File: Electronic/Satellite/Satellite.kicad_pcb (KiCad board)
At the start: 4 copper layers, 40 x 40 mm, 119 parts, among them J3 Conn_01x10, J4 Conn_01x10, J5 Conn_01x10, SW1 TS-1088-AR02016, SW2 TS-1088-AR02016, U1 LAN8651B1-E/LMX, U2 AVRH10C221KT1R5YA8, U3 AVRH10C221KT1R5YA8, U4 SY8513FCC, U5 ABM8-272-T3_C20625731, U6 NCP1117ST33T3G, U7 RP2354A, U8 WS2812C-2020-V6, X1 ABM10-25.000MHZ-D30-T3

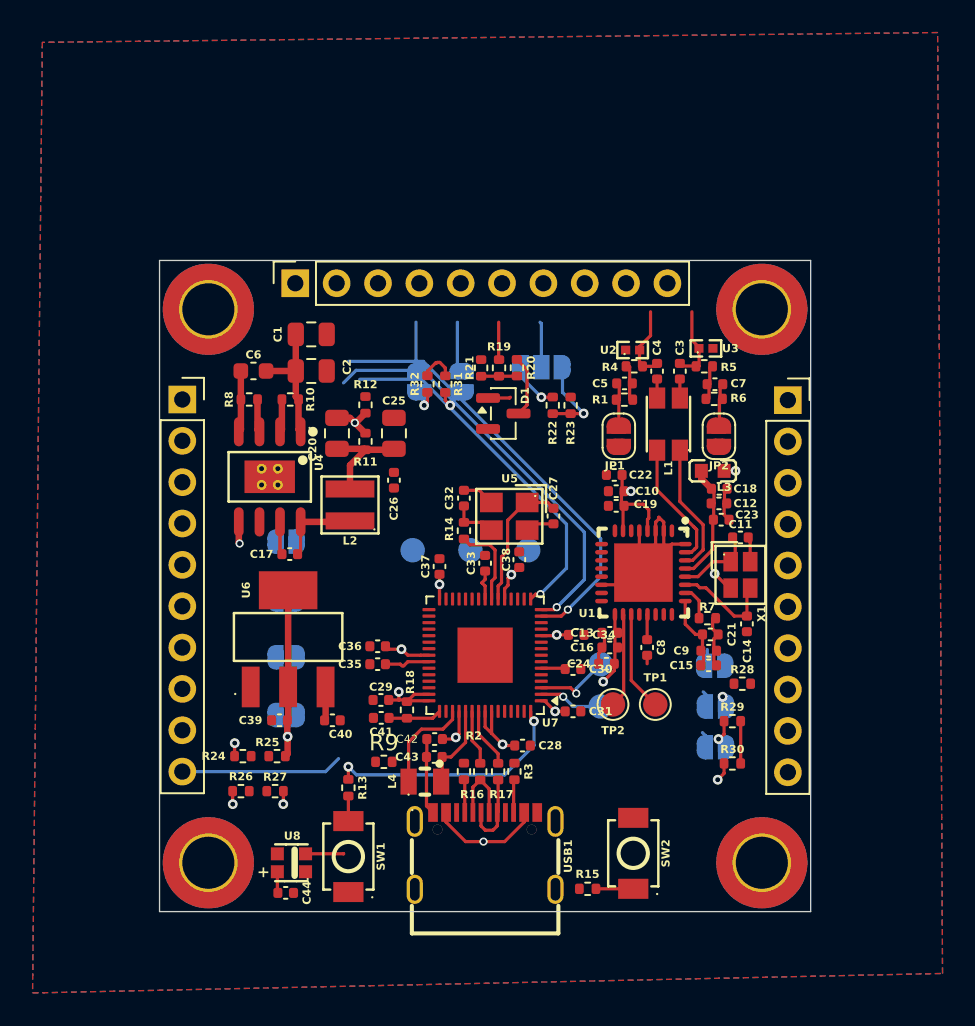
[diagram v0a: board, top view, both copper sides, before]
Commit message: Satellite PCB done !!!!!! (need verification)
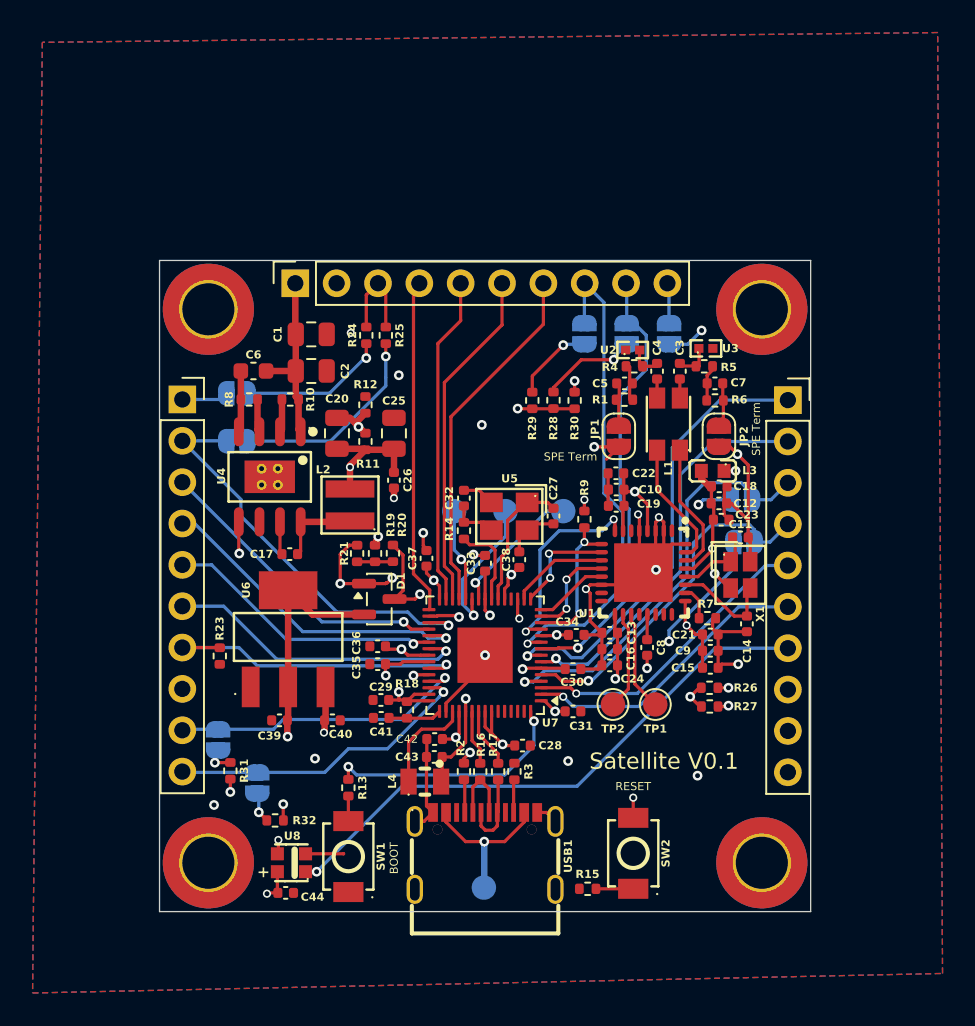
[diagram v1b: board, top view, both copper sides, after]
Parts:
- removed JP4: Jumper_3_Open, Jumper:SolderJumper-3_P1.3mm_Open_RoundedPad1.0x1.5mm
- removed R22: 4.7K, Resistor_SMD:R_0402_1005Metric
- removed TP7: TP, TestPoint:TestPoint_Pad_D1.5mm
- R23: value 9.1K -> 10K
- moved JP8 30.1 mm to (157.3, 108.5)
- moved JP7 29.6 mm to (157.2, 105.9)
- moved R26 29.5 mm to (155.2, 117.5)
- moved R32 28.4 mm to (128.5, 125.6), turned to 0 degrees
- moved R27 27.2 mm to (155.2, 118.6), turned to 180 degrees
- moved R31 27.2 mm to (125.8, 122.5), turned to -90 degrees
- moved R24 26.9 mm to (134.1, 95.8), turned to 90 degrees
- moved R25 26.7 mm to (135.3, 95.8), turned to 90 degrees
- moved JP12 26.6 mm to (125.0, 120.7)
- moved JP13 26.6 mm to (127.4, 123.3)
- moved R23 26.5 mm to (125.1, 115.5), turned to 90 degrees
- moved JP11 25.6 mm to (152.7, 95.7), turned to -90 degrees
- moved R30 24.3 mm to (146.9, 99.8), turned to -90 degrees
- moved JP10 24.3 mm to (147.5, 95.7), turned to -90 degrees
- moved R29 23.2 mm to (144.3, 99.8), turned to -90 degrees
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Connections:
- J3 pad 10: GND -> /GPIO8
- J3 pad 2: /5V -> +5V
- J3 pad 4: unconnected-(J3-Pin_4-Pad4) -> /SPI0_TX
- J3 pad 5: unconnected-(J3-Pin_5-Pad5) -> /SPI0_SCK
- J3 pad 6: unconnected-(J3-Pin_6-Pad6) -> /GPIO17
- J3 pad 7: unconnected-(J3-Pin_7-Pad7) -> /SPI0_RX
- J3 pad 8: unconnected-(J3-Pin_8-Pad8) -> /GPIO7
- J3 pad 9: /ADC3 -> /GPIO6
- J4 pad 10: /ADC2 -> /ADC3
- J4 pad 3: /I2C1_SDA -> /GPIO22
- J4 pad 4: /I2C1_SCL -> /GPIO23
- J4 pad 5: /LED_Data_Out -> /GPIO24
- J4 pad 6: /UART1_TX -> /GPIO25
- J4 pad 7: /UART1_RX -> /ADC0
- J4 pad 9: Net-(J4-Pin_9) -> /ADC2
- J5 pad 1: /GPIO6 -> /UART1_RX
- J5 pad 2: /GPIO7 -> /UART1_TX
- J5 pad 3: /GPIO8 -> /I2C1_SDA
- J5 pad 4: /RS232_TX -> /I2C1_SCL
- J5 pad 5: /RS232_TX -> /UART0_RX
- J5 pad 6: /SPI0_RX -> /UART0_TX
- J5 pad 7: /GPIO17 -> /LED_Data_Out
- J5 pad 8: /SPI0_SCK -> GND
- J5 pad 9: /SPI0_TX -> GND
- R19 pad 2: Net-(J4-Pin_9) -> Net-(J4-Pin_8)
- TP6 pad 1: /UART0_TX -> VBUS
- U7 pad 34: /CAN_INT0 -> /GPIO22
- U7 pad 35: /CAN_INT1 -> /GPIO23
- U7 pad 36: /CAN_CS -> /GPIO24
- U7 pad 37: /PWM_COB -> /GPIO25
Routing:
- net GND: track 43.4 -> 85.9 mm, vias 1 -> 23
- net /LED_Data_Out: track 0.00 -> 35.3 mm, vias 0 -> 1
- net VBUS: track 42.1 -> 9.81 mm
- net +5V: track 8.47 -> 40.6 mm, vias 0 -> 2
- net /GPIO7: track 0.00 -> 30.2 mm
- net /RUN: track 0.00 -> 30.2 mm, vias 0 -> 2
- net /I2C0_SDA: track 0.00 -> 28.3 mm, vias 0 -> 1
- net /UART1_RX: track 0.00 -> 28.1 mm, vias 0 -> 1
- net /GPIO6: track 0.00 -> 27.6 mm, vias 0 -> 1
- net /LED_Data: track 0.00 -> 26.4 mm, vias 0 -> 2
- net /I2C1_SDA: track 0.00 -> 26.1 mm, vias 0 -> 1
- net /I2C0_SCL: track 0.00 -> 25.7 mm, vias 0 -> 1
- net /UART1_TX: track 0.00 -> 24.5 mm, vias 0 -> 1
- net /SPI0_RX: track 0.00 -> 22.0 mm
- net /I2C1_SCL: track 0.00 -> 21.9 mm, vias 0 -> 1
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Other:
- board text added: "ADC2 PULLUP"
- board text added: "ADC3 PULLUP"
- board text added: "BOOT"
- board text added: "I2C0 PULLUP"
- board text added: "I2C1 PULLUP"
- board text added: "PULLUP"
- board text added: "RESET"
- board text added: "RUN"
- board text added: "SPE Term"
- board text added: "SWCLK"
- board text added: "SWDIO"
- board text added: "Satellite V0.1"
- board text added: "VBUS"
